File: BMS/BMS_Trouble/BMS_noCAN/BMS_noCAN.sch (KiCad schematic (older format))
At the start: 8 parts

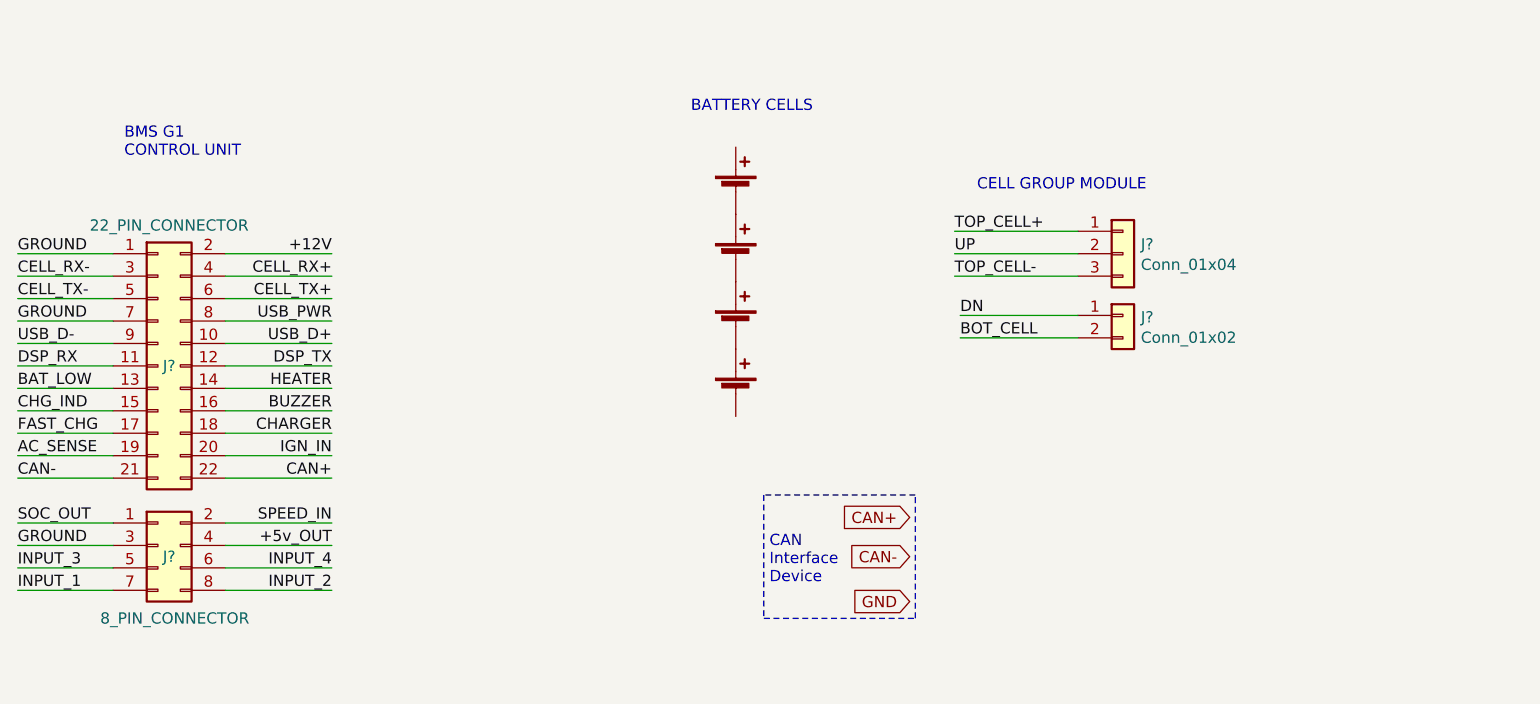
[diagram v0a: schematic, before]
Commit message: final schem
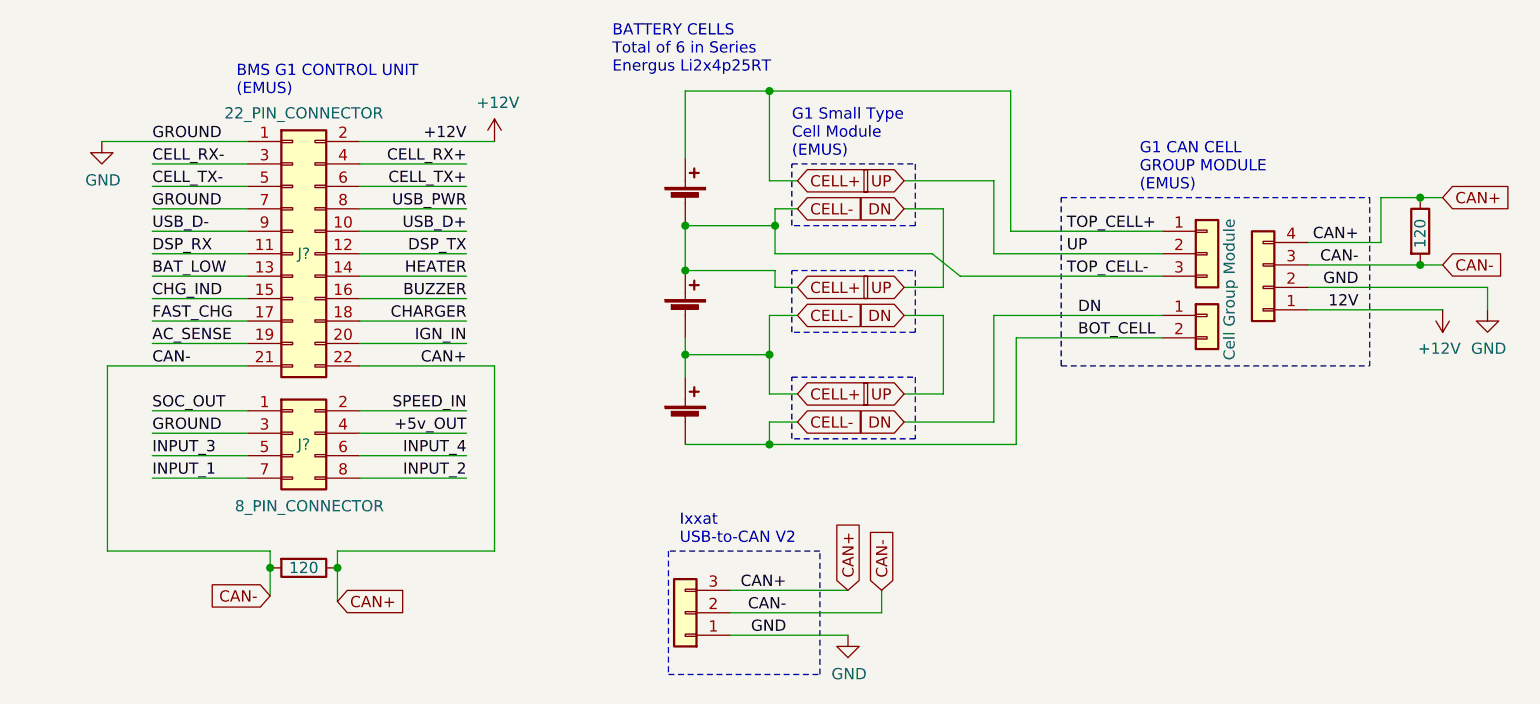
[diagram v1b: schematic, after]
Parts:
- removed BT?: Battery_Cell, symbol Device:Battery_Cell
- added J?: Conn_01x04, symbol Connector_Generic:Conn_01x04
- added J?: Conn_01x03, symbol Connector_Generic:Conn_01x03
- added R? (x2): 120, symbol Device:R
- J?: value Conn_01x04 -> Cell Group Module
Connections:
- net BOT_CELL is gone; now on net CELL+: J?.2 (Pin_2)
- net GROUND is gone; now on net GND: J?.1 (Pin_1), J?.3 (Pin_3), J?.7 (Pin_7)
- net TOP_CELL+ is gone; now on net CELL+: J?.1 (Pin_1)
- net TOP_CELL- is gone; now on net CELL+: J?.3 (Pin_3)
- net UP is gone; now on net DN: J?.2 (Pin_2)
- net +12V: now also J?.1 (Pin_1)
- net CAN+: now also J?.3 (Pin_3), J?.4 (Pin_4), R?.1, R?.1
- net CAN-: now also J?.2 (Pin_2), J?.3 (Pin_3), R?.2, R?.2
- net GND: now also J?.1 (Pin_1), J?.2 (Pin_2)
- net CELL+: now reaches BT?.1 (+)
- net CELL+: now also BT?.1 (+), BT?.1 (+), BT?.2 (-), BT?.2 (-), BT?.2 (-)
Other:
- note added: "BATTERY CELLS\nTotal of 6 in Series\nEnergus Li2x4p25RT"
- note added: "BMS G1 CONTROL UNIT\n(EMUS)"
- note added: "G1 CAN CELL \nGROUP MODULE\n(EMUS)"
- note added: "G1 Small Type\nCell Module\n(EMUS)"
- note added: "Ixxat \nUSB-to-CAN V2"
- note removed: "BATTERY CELLS"
- note removed: "BMS G1\nCONTROL UNIT"
- note removed: "CAN \nInterface\nDevice"
- note removed: "CELL GROUP MODULE\n"
- moved on the sheet: J?
